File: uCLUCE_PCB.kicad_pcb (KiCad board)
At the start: 2 copper layers, 3 parts, among them P1 USB_A, U1 PIC16F1455-I/ST, U2 MCP2003B

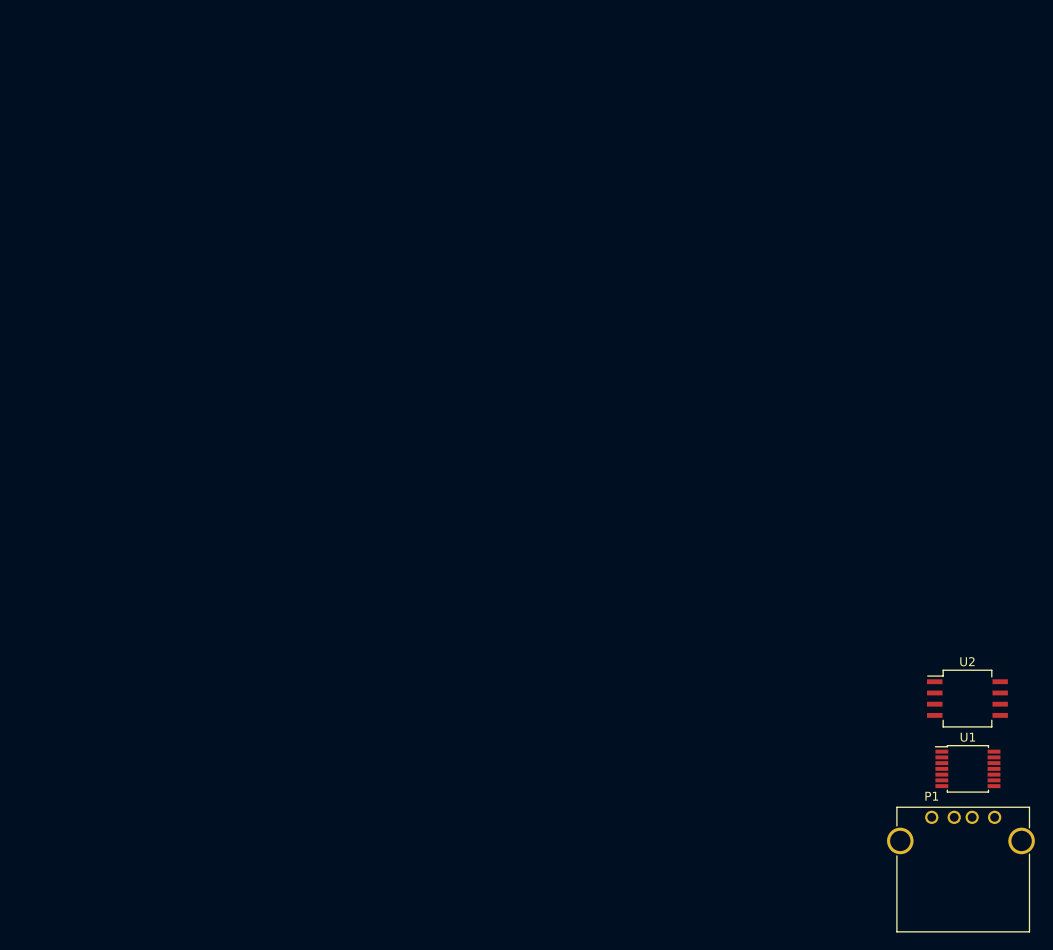
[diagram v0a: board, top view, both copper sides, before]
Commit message: Coponents add
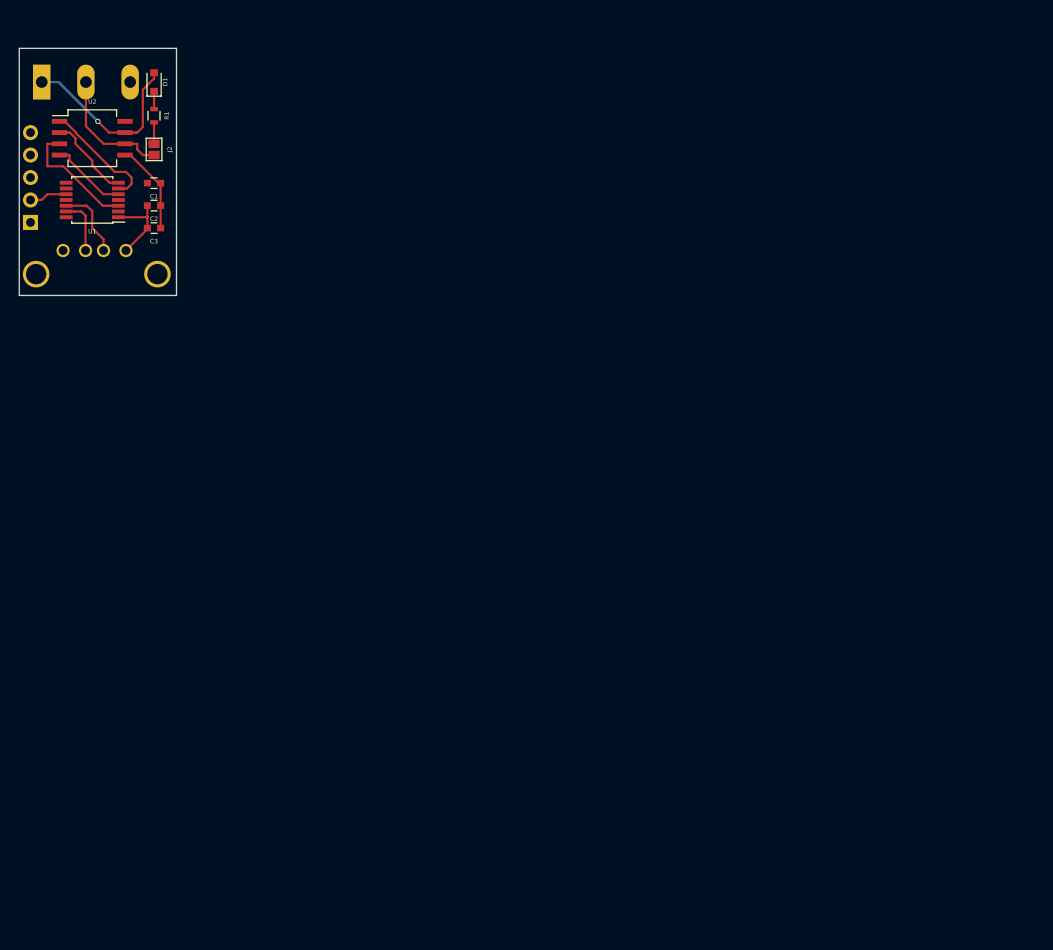
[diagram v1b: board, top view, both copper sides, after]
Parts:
- added C1: 0.47u, Capacitors_SMD:C_0603, F.Cu at (54.6, 41.9)
- added C2: 100n, Capacitors_SMD:C_0603, F.Cu at (54.6, 44.5)
- added C3: 100n, Capacitors_SMD:C_0603, F.Cu at (54.6, 47.0)
- added D1: D, Diodes_SMD:D_0805, F.Cu at (54.6, 30.5)
- added ICS1: Conn_01x05, Pin_Headers:Pin_Header_Straight_1x05_Pitch2.54mm, B.Cu at (40.6, 46.4)
- added J1: Screw_Terminal_01x03, Connectors:AK300-3, B.Cu at (41.9, 30.5)
- added J2: GS2, Connectors:GS2, F.Cu at (54.6, 38.1)
- added R1: 1k, Resistors_SMD:R_0603, F.Cu at (54.6, 34.3)
- P1: moved to B.Cu
- moved U1 118.1 mm to (47.6, 43.8), turned to 180 degrees
- moved U2 117.5 mm to (47.6, 36.8)
- moved P1 111.4 mm to (51.4, 49.5), turned to 180 degrees
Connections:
- P1 pad 1: (no net) -> +5V
- P1 pad 2: (no net) -> Net-(P1-Pad2)
- P1 pad 3: (no net) -> Net-(P1-Pad3)
- P1 pad 4: (no net) -> GND
- P1 pad 5: Net-(P1-Pad5) -> GND
- U1 pad 1: (no net) -> +5V
- U1 pad 10: (no net) -> Net-(ICS1-Pad2)
- U1 pad 11: (no net) -> Net-(C1-Pad2)
- U1 pad 12: (no net) -> Net-(P1-Pad2)
- U1 pad 13: (no net) -> Net-(P1-Pad3)
- U1 pad 14: (no net) -> GND
- U1 pad 2: (no net) -> Net-(U1-Pad2)
- U1 pad 3: (no net) -> Net-(U1-Pad3)
- U1 pad 4: (no net) -> /MCLR
- U1 pad 5: (no net) -> Net-(U1-Pad5)
- U1 pad 6: (no net) -> Net-(U1-Pad6)
- U1 pad 7: (no net) -> Net-(U1-Pad7)
- U1 pad 8: (no net) -> Net-(U1-Pad8)
- U1 pad 9: (no net) -> Net-(ICS1-Pad1)
- U2 pad 1: (no net) -> Net-(U1-Pad6)
- U2 pad 2: (no net) -> Net-(U1-Pad7)
- U2 pad 3: (no net) -> Net-(U1-Pad3)
- U2 pad 4: (no net) -> Net-(U1-Pad5)
- U2 pad 5: (no net) -> GND
- U2 pad 6: (no net) -> Net-(J1-Pad2)
- U2 pad 7: (no net) -> +BATT
- U2 pad 8: (no net) -> Net-(U2-Pad8)
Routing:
- net +BATT: track 0.00 -> 20.7 mm, vias 0 -> 1
- net Net-(J1-Pad2): track 0.00 -> 14.4 mm
- net Net-(U1-Pad3): track 0.00 -> 13.8 mm
- net Net-(U1-Pad6): track 0.00 -> 13.2 mm
- net GND: track 0.00 -> 10.4 mm
- net Net-(U1-Pad7): track 0.00 -> 9.69 mm
- net +5V: track 0.00 -> 9.39 mm
- net Net-(U1-Pad5): track 0.00 -> 8.84 mm
- net Net-(P1-Pad2): track 0.00 -> 8.83 mm
- net Net-(P1-Pad3): track 0.00 -> 6.32 mm
- net Net-(ICS1-Pad2): track 0.00 -> 4.30 mm
- net Net-(J2-Pad1): track 0.00 -> 2.42 mm
- net Net-(D1-Pad1): track 0.00 -> 2.01 mm
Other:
- board outline added: 17.8 x 27.9 mm

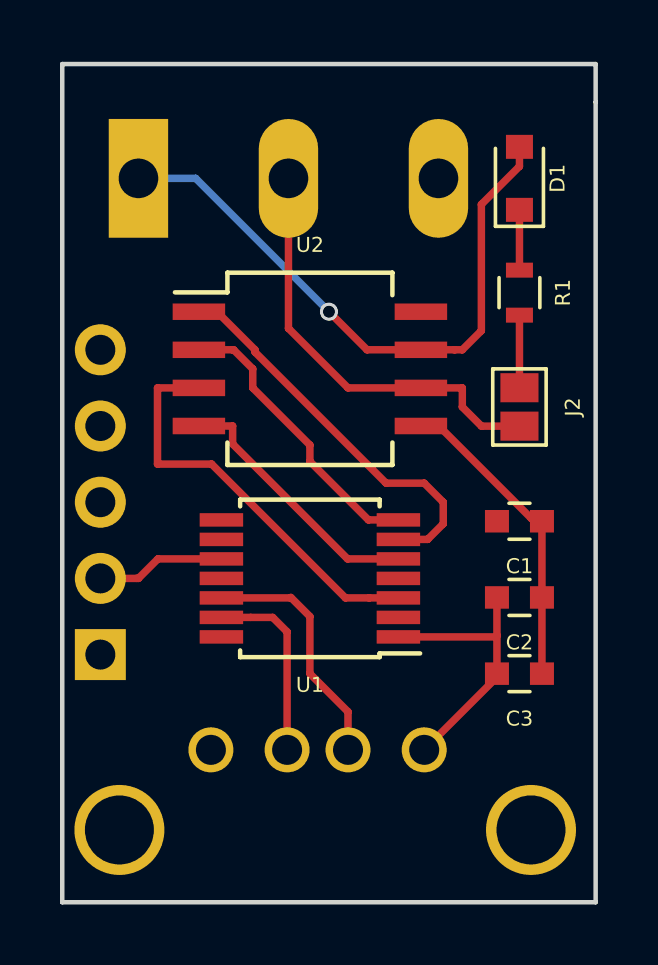
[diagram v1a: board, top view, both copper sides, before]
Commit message: Route
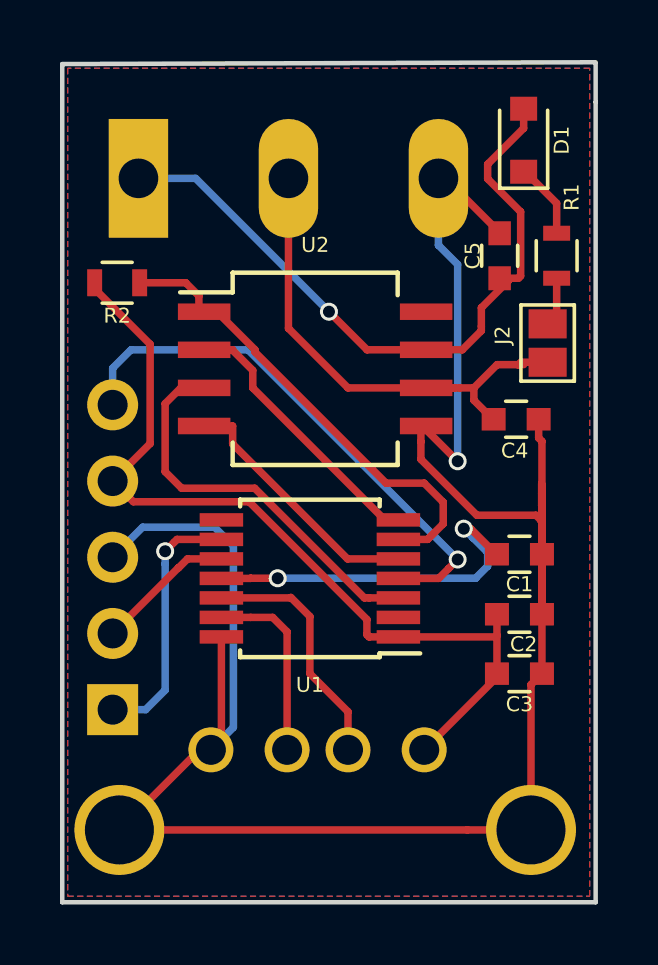
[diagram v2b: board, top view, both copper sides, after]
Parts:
- added C4: 220p, Capacitors_SMD:C_0603, F.Cu at (54.5, 38.5)
- added C5: 1u, Capacitors_SMD:C_0603, F.Cu at (54.0, 33.1)
- added R2: 4,7k, Resistors_SMD:R_0603, F.Cu at (41.2, 34.0)
- C2: value 100n -> 470n
- moved J2 2.33 mm to (55.5, 36.0)
- moved ICS1 1.88 mm to (41.0, 48.2)
- moved R1 1.75 mm to (55.9, 33.1)
- moved D1 1.28 mm to (54.8, 29.2)
- moved C1 1.10 mm to (54.6, 43.0)
- moved C2 0.56 mm to (54.6, 45.0)
- moved U2 0.17 mm to (47.8, 36.8)
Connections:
- U1 pad 2: Net-(U1-Pad2) -> (no net)
- U1 pad 8: Net-(U1-Pad8) -> (no net)
- U2 pad 8: Net-(U2-Pad8) -> (no net)
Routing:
- net GND: track 10.4 -> 76.3 mm, vias 0 -> 1
- net +5V: track 9.39 -> 28.7 mm
- net /MCLR: track 0.00 -> 18.1 mm, vias 0 -> 1
- net Net-(C1-Pad2): track 0.12 -> 12.1 mm, vias 0 -> 2
- net Net-(ICS1-Pad1): track 0.00 -> 8.69 mm, vias 0 -> 1
- net Net-(C4-Pad2): track 14.4 -> 17.3 mm
- net Net-(R2-Pad1): track 13.2 -> 15.9 mm
- net +BATT: track 20.7 -> 23.4 mm
- net Net-(J2-Pad1): track 2.42 -> 1.64 mm
- net Net-(U1-Pad3): track 13.8 -> 13.1 mm
- net Net-(D1-Pad1): track 2.01 -> 2.53 mm
- added copper zone on B.Cu, net GND
- added copper zone on F.Cu, net GND
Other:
- board size 17.8 x 27.9 mm -> 17.8 x 28 mm
- board text added: "BAT"
- board text added: "CAN DEVICES"
- board text added: "GND"
- board text added: "LIN"
- board text added: "LUC 0.1"
- board text added: "U"

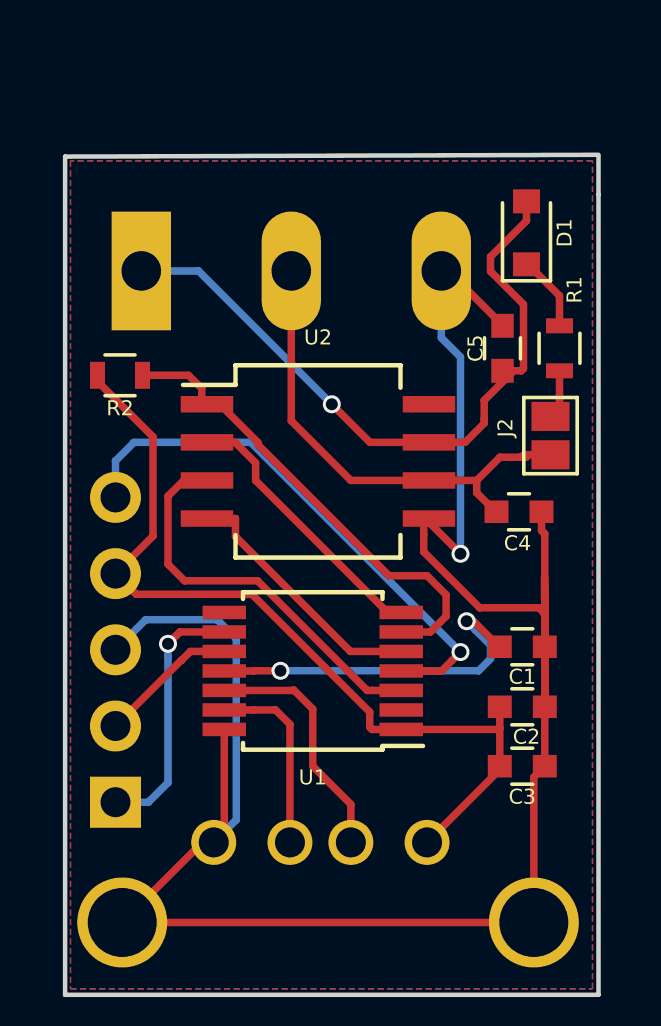
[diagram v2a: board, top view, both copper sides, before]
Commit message: diodes add
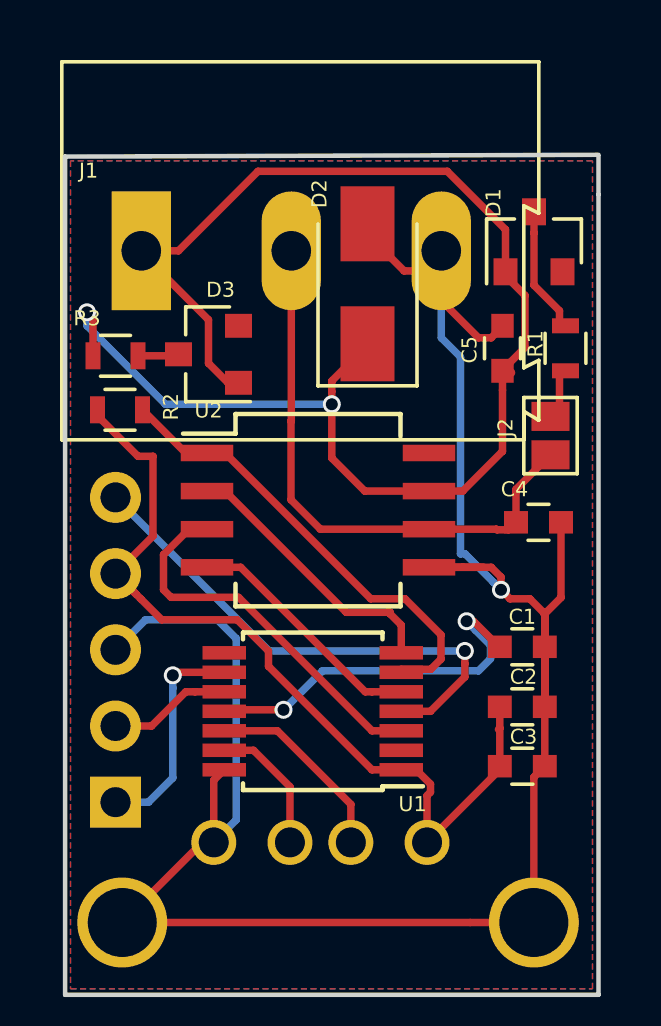
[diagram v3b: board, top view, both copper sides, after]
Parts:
- added D2: D_Schottky_Small, Diodes_SMD:D_SMA, F.Cu at (49.5, 30.9)
- added D3: SMBD914E6327HTSA1, Diodes_SMD:D_SOT-23_ANK, F.Cu at (44.1, 33.3)
- added R3: 50, Resistors_SMD:R_0603, F.Cu at (41.0, 33.3)
- D1: value D -> SMBD914E6327HTSA1; footprint Diodes_SMD:D_0805 -> Diodes_SMD:D_SOT-23_ANK
- J1: moved to F.Cu
- moved U2 1.62 mm to (47.8, 38.5)
- moved U1 1.34 mm to (47.6, 45.2)
- moved R2 1.15 mm to (41.2, 35.1)
- moved C4 0.74 mm to (55.1, 38.9), turned to 0 degrees
- moved J1 0.67 mm to (41.9, 29.8)
- moved D1 0.39 mm to (55.0, 29.5)
- moved R1 0.20 mm to (56.0, 33.1)
- turned C5 to 90 degrees
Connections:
- C4 pad 1: GND -> Net-(C4-Pad1)
- C4 pad 2: Net-(C4-Pad2) -> GND
- C5 pad 1: GND -> Net-(C5-Pad1)
- C5 pad 2: +BATT -> GND
- J1 pad 2: Net-(C4-Pad2) -> Net-(C4-Pad1)
- J2 pad 2: Net-(C4-Pad2) -> Net-(C4-Pad1)
- U2 pad 6: Net-(C4-Pad2) -> Net-(C4-Pad1)
- U2 pad 7: +BATT -> Net-(C5-Pad1)
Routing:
- net Net-(C5-Pad1): track 0.00 -> 28.1 mm, vias 0 -> 2
- net Net-(C4-Pad1): track 0.00 -> 18.8 mm
- net Net-(C4-Pad2): track 17.3 -> 0.00 mm
- net Net-(P1-Pad3): track 6.32 -> 4.55 mm
- net Net-(P1-Pad2): track 8.83 -> 7.14 mm
- net Net-(D1-Pad1): track 2.53 -> 4.15 mm
- net Net-(D3-Pad1): track 0.00 -> 1.37 mm
- net Net-(ICS1-Pad1): track 8.69 -> 7.42 mm
- net +BATT: track 23.4 -> 22.2 mm, vias 1 -> 0
- net /MCLR: track 18.1 -> 17.2 mm
- net Net-(U1-Pad5): track 8.84 -> 8.19 mm
- net +5V: track 28.7 -> 29.3 mm
- net Net-(ICS1-Pad2): track 4.65 -> 4.10 mm
- net Net-(C1-Pad2): track 12.1 -> 12.6 mm

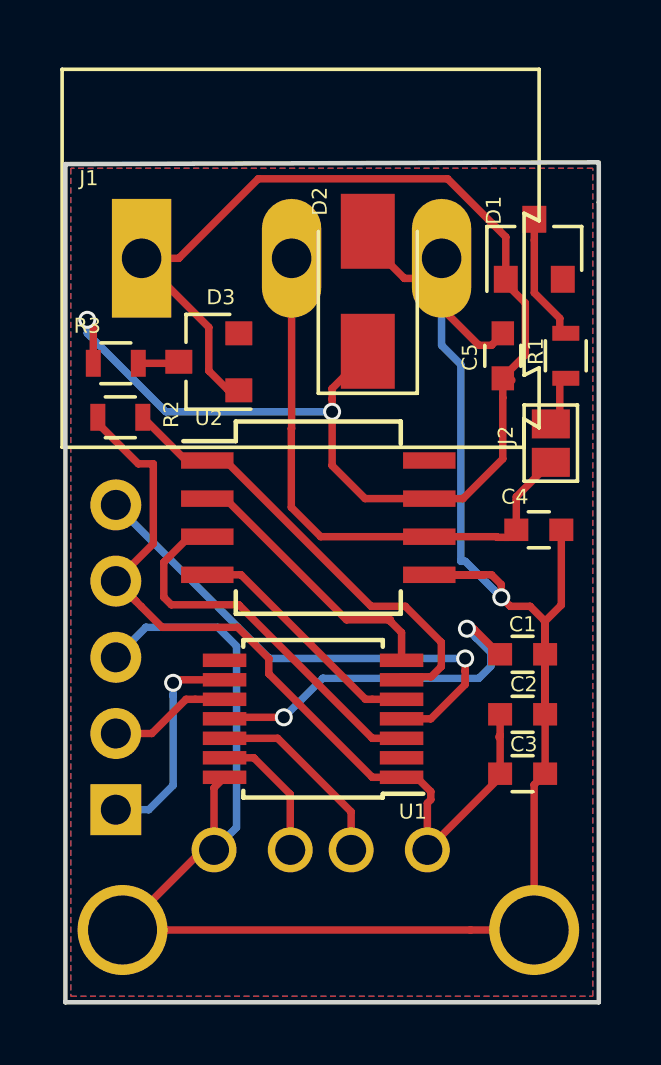
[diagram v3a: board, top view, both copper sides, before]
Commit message: Footprint update
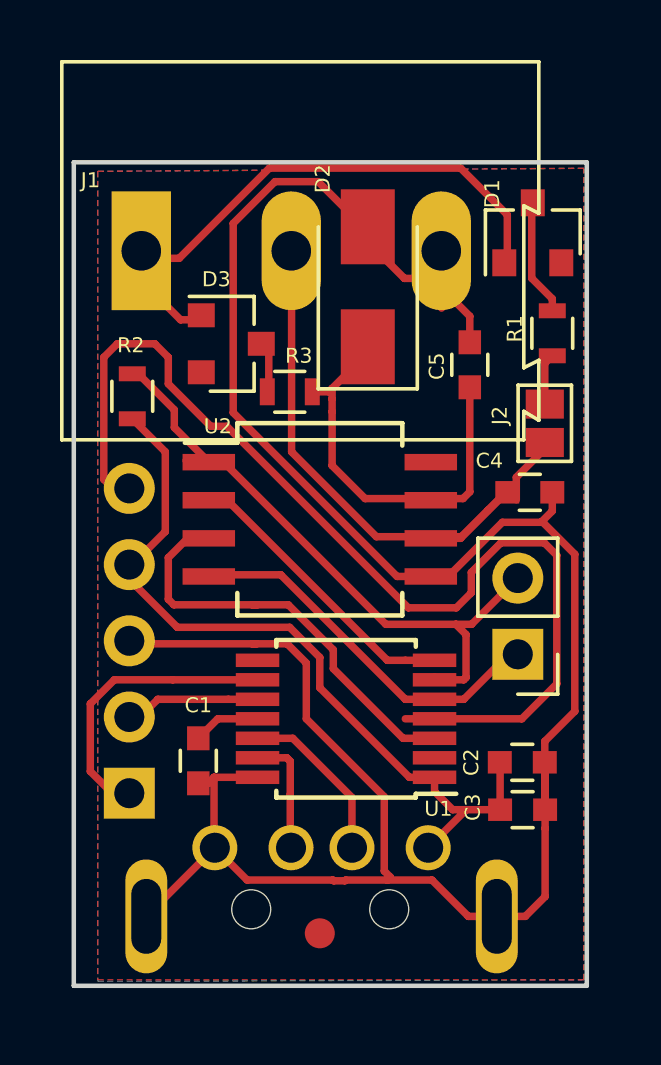
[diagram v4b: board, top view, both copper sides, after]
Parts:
- added P2: UART_TTL, Pin_Headers:Pin_Header_Straight_1x02_Pitch2.54mm, F.Cu at (54.5, 43.0)
- added U3: fiducial, Fiducials:Fiducial_1mm_Dia_2.54mm_Outer_CopperBottom, B.Cu at (47.9, 52.3)
- P1: footprint Connect:USB_A -> uCLUCE_PCB:USB_A_DS1097
- moved C1 11.4 mm to (43.8, 46.6), turned to 90 degrees
- moved R3 5.88 mm to (46.9, 34.3), turned to 180 degrees
- moved C2 1.60 mm to (54.6, 46.6)
- moved C4 1.29 mm to (54.9, 37.6)
- moved C3 1.20 mm to (54.6, 48.2)
- moved C5 1.14 mm to (52.9, 33.4)
- moved U1 1.10 mm to (48.7, 45.2)
- moved D3 0.96 mm to (44.9, 32.7), turned to 0 degrees
- moved R1 0.87 mm to (55.6, 32.3)
- moved R2 0.81 mm to (41.6, 34.4), turned to 270 degrees
- moved ICS1 0.71 mm to (41.5, 47.6)
- moved J2 0.69 mm to (55.4, 35.3)
- moved D1 0.55 mm to (55.0, 29.0)
- moved J1 0.25 mm to (41.9, 29.6)
- moved D2 0.15 mm to (49.5, 30.8)
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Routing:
- net /MCLR: track 17.2 -> 36.0 mm, vias 1 -> 0
- net Net-(C5-Pad1): track 28.1 -> 13.9 mm, vias 2 -> 0
- net Net-(C1-Pad2): track 12.6 -> 2.24 mm, vias 2 -> 0
- net GND: track 76.8 -> 87.0 mm, vias 1 -> 0
- net Net-(P2-Pad1): track 8.19 -> 13.9 mm
- net Net-(P2-Pad2): track 15.4 -> 21.1 mm
- net Net-(ICS1-Pad1): track 7.42 -> 11.1 mm, vias 1 -> 0
- net +BATT: track 22.2 -> 19.4 mm
- net Net-(U1-Pad3): track 13.4 -> 14.9 mm
- net Net-(C4-Pad1): track 18.8 -> 20.2 mm
- net +5V: track 29.3 -> 28.0 mm
- net Net-(ICS1-Pad2): track 4.10 -> 5.20 mm
- net Net-(P1-Pad2): track 7.14 -> 6.10 mm
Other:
- board size 17.8 x 28 mm -> 17.1 x 27.5 mm
- board text added: "RX"
- board text added: "TX"
